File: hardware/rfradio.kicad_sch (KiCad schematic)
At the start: 19 parts, among them U5 nRF52840

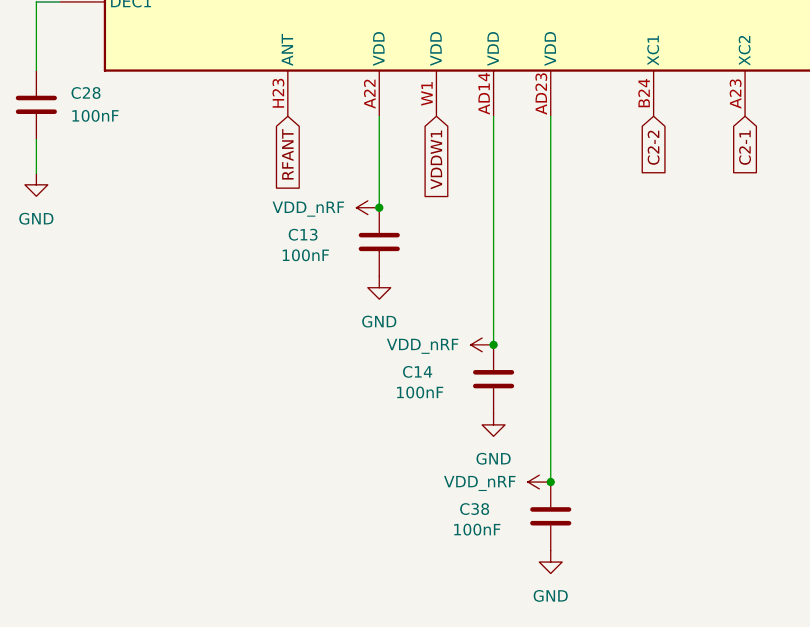
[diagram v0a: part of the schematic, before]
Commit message: all pcb routing done (i got carried away)
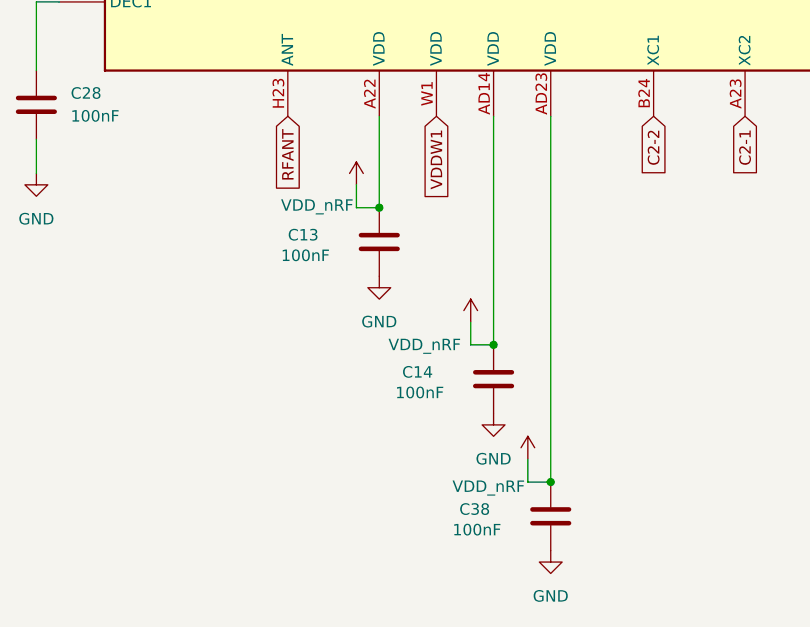
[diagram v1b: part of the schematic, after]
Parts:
- AE1: footprint (none) -> RF_Antenna:Texas_SWRA117D_2.4GHz_Left
- C13, C14, C28, C29, C30, C32, C33, C34, C35, C36, C37, C38, C39: footprint (none) -> Capacitor_SMD:C_0805_2012Metric_Pad1.18x1.45mm_HandSolder
- L1, L2, L3, L4: footprint (none) -> Inductor_SMD:L_0805_2012Metric_Pad1.05x1.20mm_HandSolder
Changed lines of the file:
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@@
 	(wire
 		(pts
+			(xy 102.87 143.51) (xy 102.87 146.05)
+		)
+		(stroke
+			(width 0)
+			(type default)
+		)
+	)
+	(wire
+		(pts
 			(xy 26.67 115.57) (xy 26.67 118.11)
 		)
@@
 	(wire
 		(pts
+			(xy 102.87 146.05) (xy 105.41 146.05)
+		)
+		(stroke
+			(width 0)
+			(type default)
+		)
+	)
+	(wire
+		(pts
 			(xy 55.88 120.65) (xy 55.88 130.81)
 		)
@@
 	(wire
 		(pts
+			(xy 115.57 161.29) (xy 118.11 161.29)
+		)
+		(stroke
+			(width 0)
+			(type default)
+		)
+	)
+	(wire
+		(pts
 			(xy 217.17 100.33) (xy 217.17 97.79)
 		)
@@
 	(wire
 		(pts
+			(xy 115.57 158.75) (xy 115.57 161.29)
+		)
+		(stroke
+			(width 0)
+			(type default)
+		)
+	)
+	(wire
+		(pts
 			(xy 67.31 138.43) (xy 67.31 142.24)
 		)
@@
 	(wire
 		(pts
+			(xy 121.92 173.99) (xy 121.92 176.53)
+		)
+		(stroke
+			(width 0)
+			(type default)
+		)
+	)
+	(wire
+		(pts
 			(xy 43.18 118.11) (xy 43.18 130.81)
 		)
@@
 	(wire
 		(pts
+			(xy 121.92 176.53) (xy 124.46 176.53)
+		)
+		(stroke
+			(width 0)
+			(type default)
+		)
+	)
+	(wire
+		(pts
 			(xy 67.31 38.1) (xy 77.47 38.1)
 		)
@@
 			)
 		)
-		(property "Footprint" ""
+		(property "Footprint" "Inductor_SMD:L_0805_2012Metric_Pad1.05x1.20mm_HandSolder"
 			(at 207.01 153.67 0)
 			(effects
@@
 			)
 		)
-		(property "Footprint" ""
+		(property "Footprint" "Capacitor_SMD:C_0805_2012Metric_Pad1.18x1.45mm_HandSolder"
 			(at 27.6352 115.57 0)
 			(effects
@@
 			)
 		)
-		(property "Footprint" ""
+		(property "Footprint" "Capacitor_SMD:C_0805_2012Metric_Pad1.18x1.45mm_HandSolder"
 			(at 16.2052 110.49 0)
 			(effects
@@
 			)
 		)
-		(property "Footprint" ""
+		(property "Footprint" "Capacitor_SMD:C_0805_2012Metric_Pad1.18x1.45mm_HandSolder"
 			(at 106.3752 153.67 0)
 			(effects
@@
 			)
 		)
-		(property "Footprint" ""
+		(property "Footprint" "Capacitor_SMD:C_0805_2012Metric_Pad1.18x1.45mm_HandSolder"
 			(at 56.8452 138.43 0)
 			(effects
@@
 			)
 		)
-		(property "Footprint" ""
+		(property "Footprint" "Capacitor_SMD:C_0805_2012Metric_Pad1.18x1.45mm_HandSolder"
 			(at 125.4252 184.15 0)
 			(effects
@@
 	(symbol
 		(lib_id "power:+3.3V")
-		(at 118.11 161.29 90)
+		(at 115.57 158.75 0)
 		(unit 1)
 		(exclude_from_sim no)
@@
 		(on_board yes)
 		(dnp no)
-		(fields_autoplaced yes)
 		(property "Reference" "#PWR031"
-			(at 121.92 161.29 0)
+			(at 115.57 162.56 0)
 			(effects
 				(font
@@
 		)
 		(property "Value" "VDD_nRF"
-			(at 114.3 161.2899 90)
+			(at 106.426 161.29 0)
 			(effects
 				(font
@@
 		)
 		(property "Footprint" ""
-			(at 118.11 161.29 0)
+			(at 115.57 158.75 0)
 			(effects
 				(font
@@
 		)
 		(property "Datasheet" ""
-			(at 118.11 161.29 0)
+			(at 115.57 158.75 0)
 			(effects
 				(font
@@
 		)
 		(property "Description" "Power symbol creates a global label with name \"+3.3V\""
-			(at 118.11 161.29 0)
+			(at 115.57 158.75 0)
 			(effects
 				(font
@@
 			)
 		)
-		(property "Footprint" ""
+		(property "Footprint" "Capacitor_SMD:C_0805_2012Metric_Pad1.18x1.45mm_HandSolder"
 			(at 233.3752 97.79 0)
 			(effects
@@
 			)
 		)
-		(property "Footprint" ""
+		(property "Footprint" "Capacitor_SMD:C_0805_2012Metric_Pad1.18x1.45mm_HandSolder"
 			(at 44.1452 138.43 0)
 			(effects
@@
 			)
 		)
-		(property "Footprint" ""
+		(property "Footprint" "Capacitor_SMD:C_0805_2012Metric_Pad1.18x1.45mm_HandSolder"
 			(at 18.7452 74.93 0)
 			(effects
@@
 	(symbol
 		(lib_id "power:+3.3V")
-		(at 105.41 146.05 90)
+		(at 102.87 143.51 0)
 		(unit 1)
 		(exclude_from_sim no)
@@
 		(on_board yes)
 		(dnp no)
-		(fields_autoplaced yes)
 		(property "Reference" "#PWR028"
-			(at 109.22 146.05 0)
+			(at 102.87 147.32 0)
 			(effects
 				(font
@@
 		)
 		(property "Value" "VDD_nRF"
-			(at 101.6 146.0499 90)
+			(at 94.488 145.796 0)
 			(effects
 				(font
@@
 		)
 		(property "Footprint" ""
-			(at 105.41 146.05 0)
+			(at 102.87 143.51 0)
 			(effects
 				(font
@@
 		)
 		(property "Datasheet" ""
-			(at 105.41 146.05 0)
+			(at 102.87 143.51 0)
 			(effects
 				(font
@@
 		)
 		(property "Description" "Power symbol creates a global label with name \"+3.3V\""
-			(at 105.41 146.05 0)
+			(at 102.87 143.51 0)
 			(effects
 				(font
@@
 			)
 		)
-		(property "Footprint" ""
+		(property "Footprint" "Inductor_SMD:L_0805_2012Metric_Pad1.05x1.20mm_HandSolder"
 			(at 63.5 38.1 0)
 			(effects
@@
 			)
 		)
-		(property "Footprint" ""
+		(property "Footprint" "Inductor_SMD:L_0805_2012Metric_Pad1.05x1.20mm_HandSolder"
 			(at 223.52 90.17 0)
 			(effects
@@
 	(symbol
 		(lib_id "power:+3.3V")
-		(at 124.46 176.53 90)
+		(at 121.92 173.99 0)
 		(unit 1)
 		(exclude_from_sim no)
@@
 		(on_board yes)
 		(dnp no)
-		(fields_autoplaced yes)
 		(property "Reference" "#PWR033"
-			(at 128.27 176.53 0)
+			(at 121.92 177.8 0)
 			(effects
 				(font
@@
 		)
 		(property "Value" "VDD_nRF"
-			(at 120.65 176.5299 90)
+			(at 113.538 177.038 0)
 			(effects
 				(font
@@
 		)
 		(property "Footprint" ""
-			(at 124.46 176.53 0)
+			(at 121.92 173.99 0)
 			(effects
 				(font
@@
 		)
 		(property "Datasheet" ""
-			(at 124.46 176.53 0)
+			(at 121.92 173.99 0)
 			(effects
 				(font
@@
 		)
 		(property "Description" "Power symbol creates a global label with name \"+3.3V\""
-			(at 124.46 176.53 0)
+			(at 121.92 173.99 0)
 			(effects
 				(font
@@
 			)
 		)
-		(property "Footprint" ""
+		(property "Footprint" "RF_Antenna:Texas_SWRA117D_2.4GHz_Left"
 			(at 243.84 90.17 0)
 			(effects
@@
 			)
 		)
-		(property "Footprint" ""
+		(property "Footprint" "Capacitor_SMD:C_0805_2012Metric_Pad1.18x1.45mm_HandSolder"
 			(at 226.06 152.7048 0)
 			(effects
@@
 			)
 		)
-		(property "Footprint" ""
+		(property "Footprint" "Capacitor_SMD:C_0805_2012Metric_Pad1.18x1.45mm_HandSolder"
 			(at 218.1352 97.79 0)
 			(effects
@@
 			)
 		)
-		(property "Footprint" ""
+		(property "Footprint" "Capacitor_SMD:C_0805_2012Metric_Pad1.18x1.45mm_HandSolder"
 			(at 32.7152 138.43 0)
 			(effects
@@
 			)
 		)
-		(property "Footprint" ""
+		(property "Footprint" "Inductor_SMD:L_0805_2012Metric_Pad1.05x1.20mm_HandSolder"
 			(at 214.63 153.67 0)
 			(effects
@@
 			)
 		)
-		(property "Footprint" ""
+		(property "Footprint" "Capacitor_SMD:C_0805_2012Metric_Pad1.18x1.45mm_HandSolder"
 			(at 119.0752 168.91 0)
 			(effects
@@
 			)
 		)
-		(property "Footprint" ""
+		(property "Footprint" "Capacitor_SMD:C_0805_2012Metric_Pad1.18x1.45mm_HandSolder"
 			(at 68.2752 138.43 0)
 			(effects
